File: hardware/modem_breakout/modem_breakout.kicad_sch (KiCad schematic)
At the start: 78 parts, among them J1 2016504-1, J2 NSIM-7-A, J3 54-00166, J4 Conn_01x02, J5 Conn_01x07, J6 Conn_01x02, Q1 BSS138, Q2 DTC043ZEBTL, Q3 DTC043ZEBTL, U1 EC25AFA-512-STD, U2 TXS0108EPWR, U3 MIC29302WU, U4 TLV320AIC3104IRHBR, U5 AMS1117-1.5, U6 AMS1117-1.5

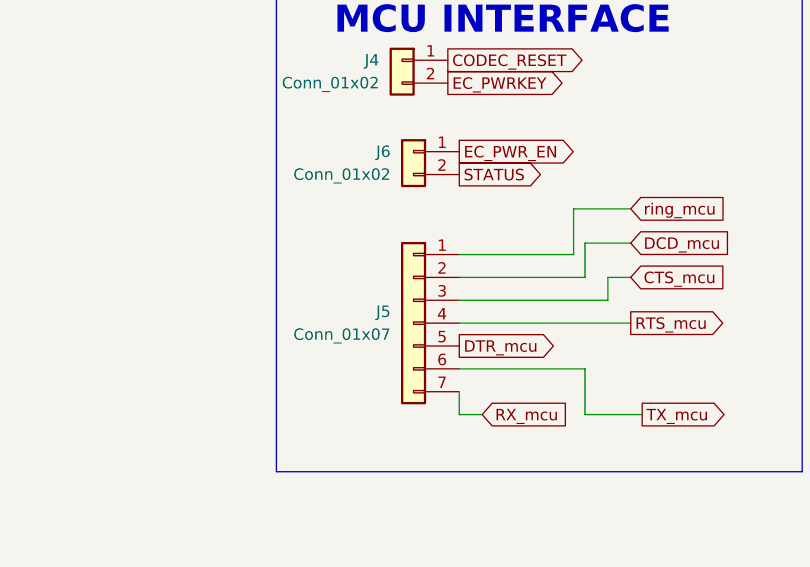
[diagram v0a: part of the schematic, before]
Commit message: final - ordered
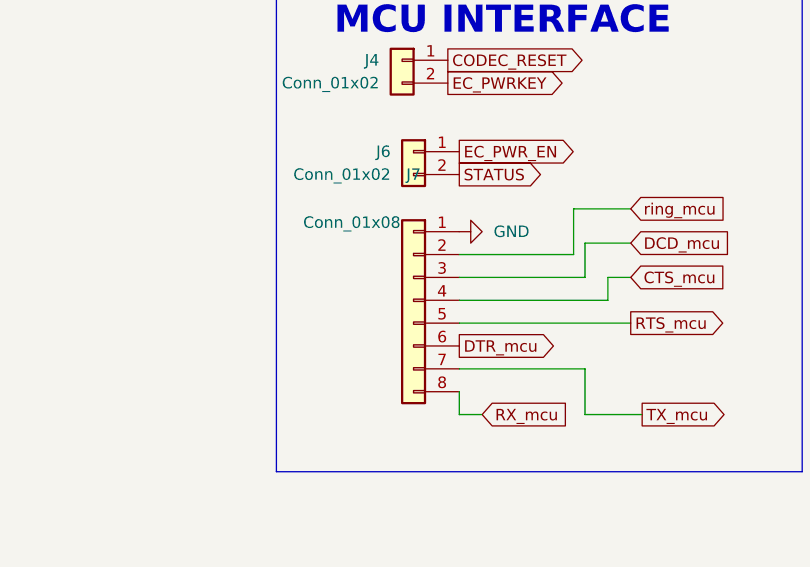
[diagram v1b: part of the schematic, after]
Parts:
- removed J5: Conn_01x07, Connector_PinHeader_2.54mm:PinHeader_1x07_P2.54mm_Vertical, symbol Connector_Generic:Conn_01x07
- added J7: Conn_01x08, Connector_PinHeader_2.54mm:PinHeader_1x08_P2.54mm_Vertical, symbol Connector_Generic:Conn_01x08
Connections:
- net CTS_mcu: now also J7.4 (Pin_4)
- net DCD_mcu: now also J7.3 (Pin_3)
- net DTR_mcu: now also J7.6 (Pin_6)
- net GND: now also J7.1 (Pin_1)
- net RTS_mcu: now also J7.5 (Pin_5)
- net RX_mcu: now also J7.8 (Pin_8)
- net TX_mcu: now also J7.7 (Pin_7)
- net ring_mcu: now also J7.2 (Pin_2)
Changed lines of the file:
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@@
 	)
 	(symbol
-		(lib_id "Connector_Generic:Conn_01x07")
-		(at 392.43 198.12 0)
-		(mirror y)
-		(unit 1)
-		(exclude_from_sim no)
-		(in_bom yes)
-		(on_board yes)
-		(dnp no)
-		(property "Reference" "J5"
-			(at 389.89 196.8499 0)
-			(effects
-				(font
-					(size 1.27 1.27)
-				)
-				(justify left)
-			)
-		)
-		(property "Value" "Conn_01x07"
-			(at 389.89 199.3899 0)
-			(effects
-				(font
-					(size 1.27 1.27)
-				)
-				(justify left)
-			)
-		)
-		(property "Footprint" "Connector_PinHeader_2.54mm:PinHeader_1x07_P2.54mm_Vertical"
-			(at 392.43 198.12 0)
-			(effects
-				(font
-					(size 1.27 1.27)
-				)
-				(hide yes)
-			)
-		)
-		(property "Datasheet" "~"
-			(at 392.43 198.12 0)
-			(effects
-				(font
-					(size 1.27 1.27)
-				)
-				(hide yes)
-			)
-		)
-		(property "Description" "Generic connector, single row, 01x07, script generated (kicad-library-utils/schlib/autogen/connector/)"
-			(at 392.43 198.12 0)
-			(effects
-				(font
-					(size 1.27 1.27)
-				)
-				(hide yes)
-			)
-		)
-		(pin "2"
-		)
-		(pin "4"
-		)
-		(pin "1"
-		)
-		(pin "6"
-		)
-		(pin "3"
-		)
-		(pin "5"
-		)
-		(pin "7"
-		)
-		(instances
-			(project ""
-				(path "/65e82cba-9b7b-4a65-9f94-7e409cc8dcd9"
-					(reference "J5")
-					(unit 1)
-				)
-			)
-		)
-	)
-	(symbol
 		(lib_id "Device:R")
 		(at 759.46 542.29 90)
@@
 	)
 	(symbol
+		(lib_id "Connector_Generic:Conn_01x08")
+		(at 392.43 195.58 0)
+		(mirror y)
+		(unit 1)
+		(exclude_from_sim no)
+		(in_bom yes)
+		(on_board yes)
+		(dnp no)
+		(property "Reference" "J7"
+			(at 392.43 181.61 0)
+			(effects
+				(font
+					(size 1.27 1.27)
+				)
+			)
+		)
+		(property "Value" "Conn_01x08"
+			(at 385.572 186.944 0)
+			(effects
+				(font
+					(size 1.27 1.27)
+				)
+			)
+		)
+		(property "Footprint" "Connector_PinHeader_2.54mm:PinHeader_1x08_P2.54mm_Vertical"
+			(at 392.43 195.58 0)
+			(effects
+				(font
+					(size 1.27 1.27)
+				)
+				(hide yes)
+			)
+		)
+		(property "Datasheet" "~"
+			(at 392.43 195.58 0)
+			(effects
+				(font
+					(size 1.27 1.27)
+				)
+				(hide yes)
+			)
+		)
+		(property "Description" "Generic connector, single row, 01x08, script generated (kicad-library-utils/schlib/autogen/connector/)"
+			(at 392.43 195.58 0)
+			(effects
+				(font
+					(size 1.27 1.27)
+				)
+				(hide yes)
+			)
+		)
+		(pin "4"
+		)
+		(pin "6"
+		)
+		(pin "3"
+		)
+		(pin "2"
+		)
+		(pin "8"
+		)
+		(pin "5"
+		)
+		(pin "1"
+		)
+		(pin "7"
+		)
+		(instances
+			(project ""
+				(path "/65e82cba-9b7b-4a65-9f94-7e409cc8dcd9"
+					(reference "J7")
+					(unit 1)
+				)
+			)
+		)
+	)
+	(symbol
 		(lib_id "Device:R")
 		(at 521.97 317.5 270)
@@
 					(unit 1)
 				)
+			)
+		)
+	)
+	(symbol
+		(lib_id "power:GND")
+		(at 397.51 187.96 90)
+		(unit 1)
+		(exclude_from_sim no)
+		(in_bom yes)
+		(on_board yes)
+		(dnp no)
+		(fields_autoplaced yes)
+		(property "Reference" "#PWR043"
+			(at 403.86 187.96 0)
+			(effects
+				(font
+					(size 1.27 1.27)
+				)
+				(hide yes)
+			)
+		)
+		(property "Value" "GND"
+			(at 401.32 187.9599 90)
+			(effects
+				(font
+					(size 1.27 1.27)
+				)
+				(justify right)
+			)
+		)
+		(property "Footprint" ""
+			(at 397.51 187.96 0)
+			(effects
+				(font
+					(size 1.27 1.27)
+				)
+				(hide yes)
+			)
+		)
+		(property "Datasheet" ""
+			(at 397.51 187.96 0)
+			(effects
+				(font
+					(size 1.27 1.27)
+				)
+				(hide yes)
+			)
+		)
+		(property "Description" "Power symbol creates a global label with name \"GND\" , ground"
+			(at 397.51 187.96 0)
+			(effects
+				(font
+					(size 1.27 1.27)
+				)
+				(hide yes)
+			)
+		)
+		(pin "1"
+		)
+		(instances
+			(project "modem_breakout"
+				(path "/65e82cba-9b7b-4a65-9f94-7e409cc8dcd9"
+					(reference "#PWR043")
+					(unit 1)
+				)
